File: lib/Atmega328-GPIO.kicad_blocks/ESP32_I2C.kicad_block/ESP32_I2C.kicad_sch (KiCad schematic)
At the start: 23 parts, among them J10 Conn_01x04_Socket, J9 DE9_Pins, SW12 SW_DIP_x01, SW13 SW_Push, SW14 SW_Push, U4 ESP-WROOM-32D

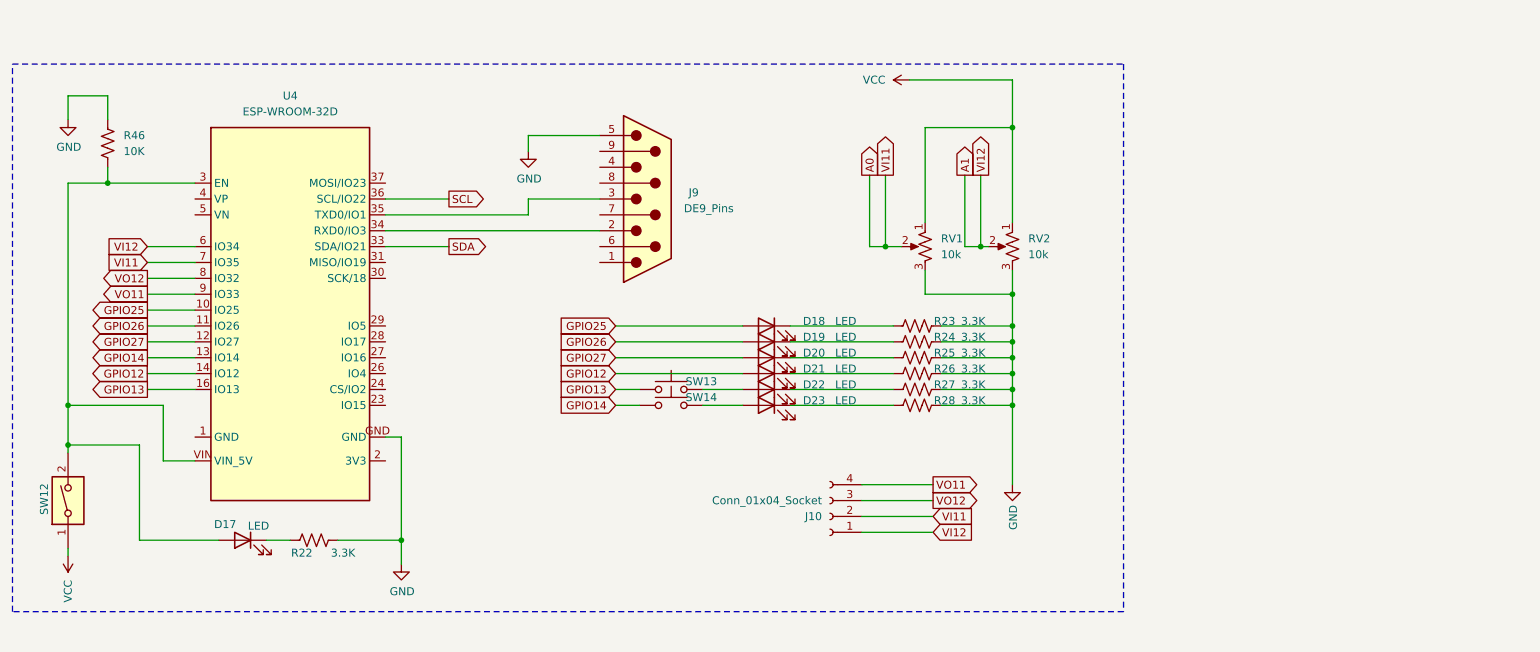
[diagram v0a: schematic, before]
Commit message: 5/21/25-1
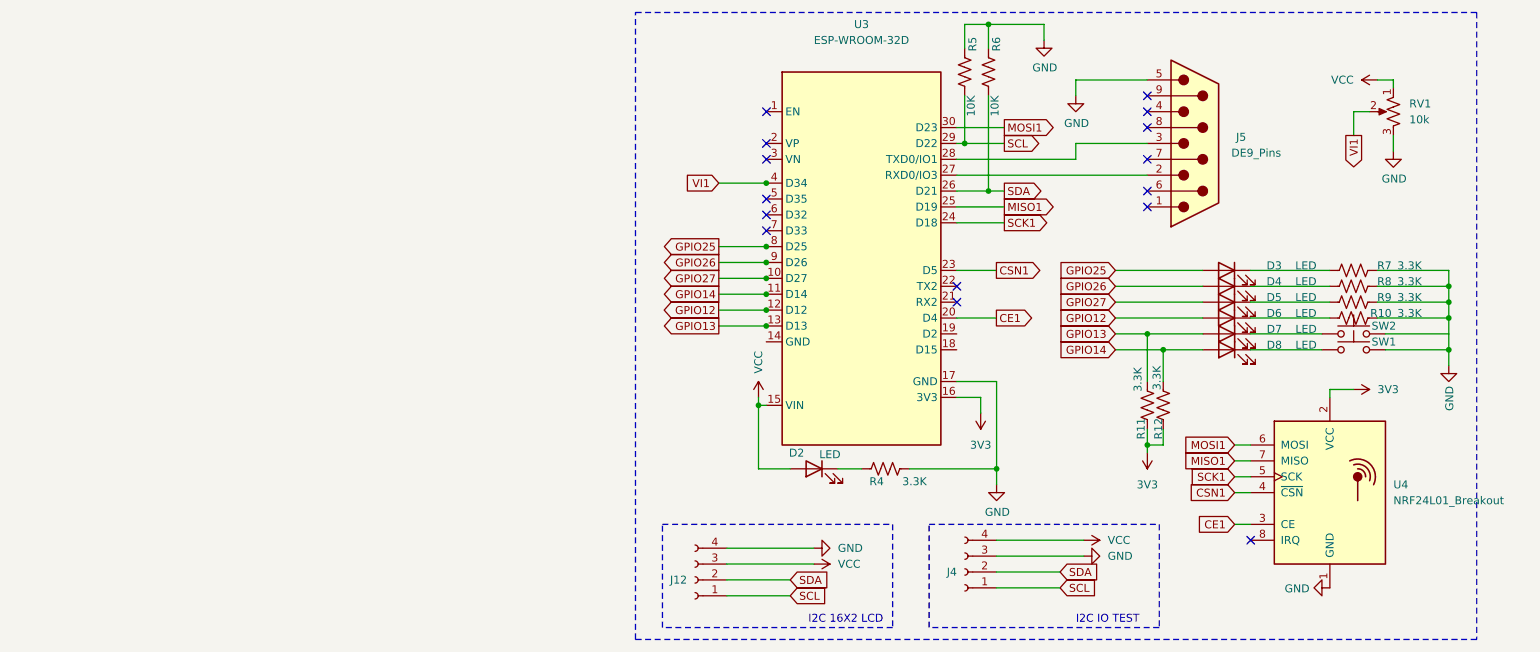
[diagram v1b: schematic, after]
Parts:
- removed D18, D23: LED, LED_THT:LED_D3.0mm_Horizontal_O1.27mm_Z2.0mm, symbol Device:LED
- removed J10: Conn_01x04_Socket, Connector_Samtec_HPM_THT:Samtec_HPM-04-01-x-S_Straight_1x04_Pitch5.08mm, symbol Connector:Conn_01x04_Socket
- removed R46: 10K, symbol Device:R_US
- removed RV2: 10k, Potentiometer_THT:Potentiometer_Alps_RK09Y11_Single_Horizontal, symbol Device:R_Potentiometer_US
- removed SW12: SW_DIP_x01, Button_Switch_THT:SW_DIP_SPSTx01_Slide_9.78x4.72mm_W7.62mm_P2.54mm, symbol Switch:SW_DIP_x01
- removed SW14: SW_Push, Button_Switch_THT:SW_DIP_SPSTx01_Slide_6.7x4.1mm_W7.62mm_P2.54mm_LowProfile, symbol Switch:SW_Push
- removed U4: ESP-WROOM-32D, symbol Add_new:ESP-WROOM-32D
- added D3, D8: LED, LED_THT:LED_D3.0mm_Horizontal_O1.27mm_Z2.0mm, symbol Device:LED
- added J12: Conn_01x04_Socket, Add_New:CONN_PPPC041LGBN-RC_SUL, symbol Connector:Conn_01x04_Socket
- added J4: Conn_01x04_Socket, Add_New:CONN_PPTC041LFBN-RC_SUL, symbol Connector:Conn_01x04_Socket
- added R5, R6: 10K, Resistor_THT:R_Axial_DIN0207_L6.3mm_D2.5mm_P10.16mm_Horizontal, symbol Device:R_US
- added SW2: SW_Push, Button_Switch_SMD:SW_Tactile_SPST_NO_Straight_CK_PTS636Sx25SMTRLFS, symbol Switch:SW_Push
- added U3: ESP-WROOM-32D, Add_New:ESP-WROOM-32D, symbol Add_new:ESP-WROOM-32D
- added U4: NRF24L01_Breakout, RF_Module:nRF24L01_Breakout, symbol RF:NRF24L01_Breakout
- R10: renamed from R26; footprint Resistor_THT:R_Axial_DIN0204_L3.6mm_D1.6mm_P5.08mm_Horizontal -> Resistor_THT:R_Axial_DIN0207_L6.3mm_D2.5mm_P10.16mm_Horizontal
- R11: renamed from R27; footprint Resistor_THT:R_Axial_DIN0204_L3.6mm_D1.6mm_P5.08mm_Horizontal -> Resistor_THT:R_Axial_DIN0207_L6.3mm_D2.5mm_P10.16mm_Horizontal
- R12: renamed from R28; footprint Resistor_THT:R_Axial_DIN0204_L3.6mm_D1.6mm_P5.08mm_Horizontal -> Resistor_THT:R_Axial_DIN0207_L6.3mm_D2.5mm_P10.16mm_Horizontal
- R4: renamed from R22; footprint Resistor_THT:R_Axial_DIN0204_L3.6mm_D1.6mm_P5.08mm_Horizontal -> Resistor_THT:R_Axial_DIN0207_L6.3mm_D2.5mm_P10.16mm_Horizontal
- R7: renamed from R23; footprint Resistor_THT:R_Axial_DIN0204_L3.6mm_D1.6mm_P5.08mm_Horizontal -> Resistor_THT:R_Axial_DIN0207_L6.3mm_D2.5mm_P10.16mm_Horizontal
- R8: renamed from R24; footprint Resistor_THT:R_Axial_DIN0204_L3.6mm_D1.6mm_P5.08mm_Horizontal -> Resistor_THT:R_Axial_DIN0207_L6.3mm_D2.5mm_P10.16mm_Horizontal
- R9: renamed from R25; footprint Resistor_THT:R_Axial_DIN0204_L3.6mm_D1.6mm_P5.08mm_Horizontal -> Resistor_THT:R_Axial_DIN0207_L6.3mm_D2.5mm_P10.16mm_Horizontal
- RV1: footprint Potentiometer_THT:Potentiometer_Alps_RK09Y11_Single_Horizontal -> Potentiometer_THT:Potentiometer_Alps_RK163_Single_Horizontal
- SW1: renamed from SW13; footprint Button_Switch_THT:SW_DIP_SPSTx01_Slide_6.7x4.1mm_W7.62mm_P2.54mm_LowProfile -> Button_Switch_SMD:SW_Tactile_SPST_NO_Straight_CK_PTS636Sx25SMTRLFS
- renumbered D17 to D2, D19 to D4, D20 to D5, D21 to D6, D22 to D7, J9 to J5
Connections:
- net GND: now also SW1.2, J12.4 (Pin_4), J4.3 (Pin_3), R5.1, R6.1, U3.17 (GND), U4.1 (GND); no longer R11.2, R12.2
- net GPIO12: now also U3.12 (D12)
- net GPIO13: now also D7.2 (A), R11.2, U3.13 (D13); no longer SW1.1
- net GPIO14: now also R12.2, D8.2 (A), U3.11 (D14)
- net GPIO25: now also D3.2 (A), U3.8 (D25)
- net GPIO26: now also U3.9 (D26)
- net GPIO27: now also U3.10 (D27)
- net SCL: now also J12.1 (Pin_1), J4.1 (Pin_1), R5.2, U3.29 (D22)
- net SDA: now also J12.2 (Pin_2), J4.2 (Pin_2), R6.2, U3.26 (D21)
- net VCC: now also D2.2 (A), J12.3 (Pin_3), J4.4 (Pin_4), U3.15 (VIN)
- net 3V3: now reaches R12.1
- net 3V3: now also R11.1, U4.2 (VCC)
- net at D7.1 (K): now also SW2.1; no longer R11.1
- net at R7.1: now also D3.1 (K)
- net at J5.2: now also U3.27 (RXD0/IO3)
- net at J5.3: now also U3.28 (TXD0/IO1)
- net A0 renamed VI1
- net VI1: now also U3.4 (D34)
- new net: D8.1 (K), SW1.1
- new net CE1: U3.20 (D4), U4.3 (CE)
- new net CSN1: U3.23 (D5), U4.4 (~{CSN})
- new net MISO1: U3.25 (D19), U4.7 (MISO)
- new net MOSI1: U3.30 (D23), U4.6 (MOSI)
- new net SCK1: U3.24 (D18), U4.5 (SCK)
- no-connect marks 0 -> 15
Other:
- note added: "I2C 16X2 LCD"
- note added: "I2C IO TEST"
- moved on the sheet: D2, D4, D5, D6, D7, J5, R10, R11, R12, R4, R7, R8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
